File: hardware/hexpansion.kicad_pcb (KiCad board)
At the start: 2 copper layers, 86 x 45.6 mm, 87 parts, among them J1 Hexpansion-Connector, U1 AP3602AKTR-G1, U10 XL-0807RGBC-WS2812B-S, U11 XL-0807RGBC-WS2812B-S, U12 XL-0807RGBC-WS2812B-S, U13 XL-0807RGBC-WS2812B-S, U14 XL-0807RGBC-WS2812B-S, U15 XL-0807RGBC-WS2812B-S, U16 XL-0807RGBC-WS2812B-S, U17 XL-0807RGBC-WS2812B-S, U18 XL-0807RGBC-WS2812B-S, U19 XL-0807RGBC-WS2812B-S, U2 ZD24C64A-XGMT, U20 XL-0807RGBC-WS2812B-S, U21 XL-0807RGBC-WS2812B-S, U22 XL-0807RGBC-WS2812B-S, U23 XL-0807RGBC-WS2812B-S, U24 XL-0807RGBC-WS2812B-S, U25 XL-0807RGBC-WS2812B-S, U26 XL-0807RGBC-WS2812B-S, U27 XL-0807RGBC-WS2812B-S, U28 XL-0807RGBC-WS2812B-S, U29 XL-0807RGBC-WS2812B-S, U3 XL-0807RGBC-WS2812B-S, U30 XL-0807RGBC-WS2812B-S, U31 XL-0807RGBC-WS2812B-S, U32 XL-0807RGBC-WS2812B-S, U33 XL-0807RGBC-WS2812B-S, U34 XL-0807RGBC-WS2812B-S, U35 XL-0807RGBC-WS2812B-S, U36 XL-0807RGBC-WS2812B-S, U37 XL-0807RGBC-WS2812B-S, U38 XL-0807RGBC-WS2812B-S, U39 XL-0807RGBC-WS2812B-S, U4 XL-0807RGBC-WS2812B-S, U40 XL-0807RGBC-WS2812B-S, U41 XL-0807RGBC-WS2812B-S, U42 XL-0807RGBC-WS2812B-S, U43 XL-0807RGBC-WS2812B-S, U44 XL-0807RGBC-WS2812B-S, U45 XL-0807RGBC-WS2812B-S, U46 XL-0807RGBC-WS2812B-S, U47 XL-0807RGBC-WS2812B-S, U48 XL-0807RGBC-WS2812B-S, U49 XL-0807RGBC-WS2812B-S, U5 XL-0807RGBC-WS2812B-S, U50 XL-0807RGBC-WS2812B-S, U51 XL-0807RGBC-WS2812B-S, U52 XL-0807RGBC-WS2812B-S, U53 XL-0807RGBC-WS2812B-S, U54 XL-0807RGBC-WS2812B-S, U55 XL-0807RGBC-WS2812B-S, U56 XL-0807RGBC-WS2812B-S, U57 XL-0807RGBC-WS2812B-S, U58 XL-0807RGBC-WS2812B-S, U59 XL-0807RGBC-WS2812B-S, U6 XL-0807RGBC-WS2812B-S, U60 XL-0807RGBC-WS2812B-S, U61 XL-0807RGBC-WS2812B-S, U62 XL-0807RGBC-WS2812B-S, U63 XL-0807RGBC-WS2812B-S, U64 XL-0807RGBC-WS2812B-S, U65 XL-0807RGBC-WS2812B-S, U66 XL-0807RGBC-WS2812B-S, U67 XL-0807RGBC-WS2812B-S, U68 XL-0807RGBC-WS2812B-S, U69 XL-0807RGBC-WS2812B-S, U7 XL-0807RGBC-WS2812B-S, U70 XL-0807RGBC-WS2812B-S, U71 XL-0807RGBC-WS2812B-S, U72 XL-0807RGBC-WS2812B-S, U73 XL-0807RGBC-WS2812B-S, U74 XL-0807RGBC-WS2812B-S, U75 XL-0807RGBC-WS2812B-S, U76 XL-0807RGBC-WS2812B-S, U77 XL-0807RGBC-WS2812B-S, U78 XL-0807RGBC-WS2812B-S, U8 XL-0807RGBC-WS2812B-S, U9 XL-0807RGBC-WS2812B-S

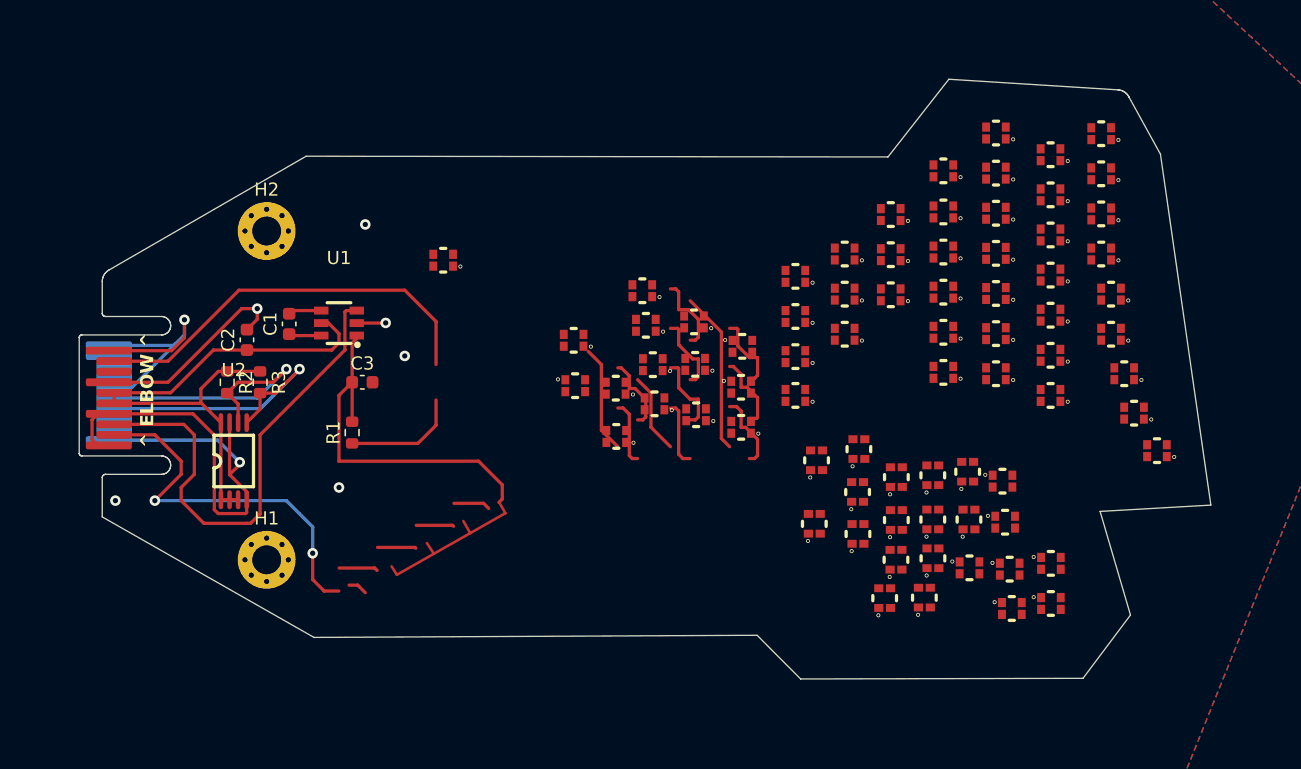
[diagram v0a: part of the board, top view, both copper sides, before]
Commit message: Fully routed
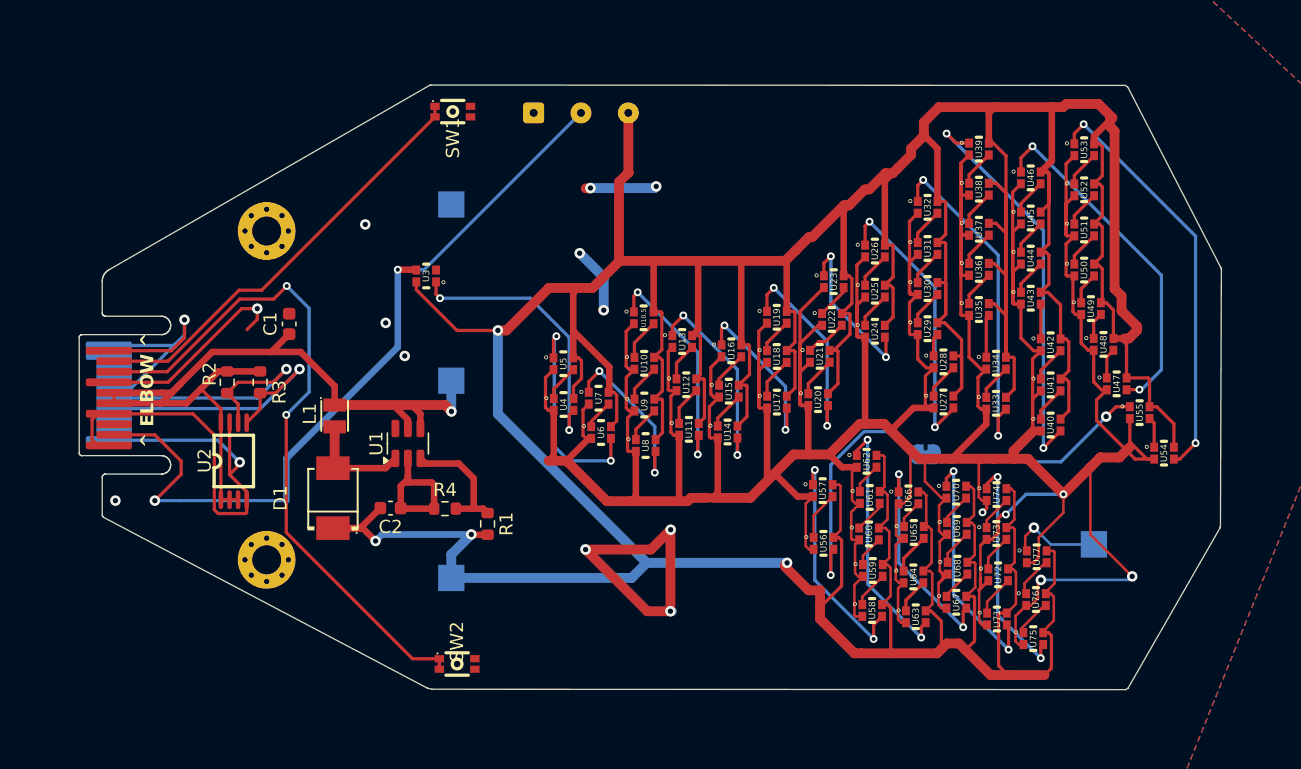
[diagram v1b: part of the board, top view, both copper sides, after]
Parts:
- removed C3: 1uF, Capacitor_SMD:C_0603_1608Metric
- added D1: SS38BF, easyeda2kicad:SMBF_L4.3-W3.6-LS5.3-RD, F.Cu at (117.5, 107.8)
- added J2: Conn_01x03_Pin, Connector_Wire:SolderWire-0.1sqmm_1x03_P3.6mm_D0.4mm_OD1mm, B.Cu at (132.8, 78.5)
- added JP1: SolderJumper_2_Bridged, Jumper:SolderJumper-2_P1.3mm_Bridged_RoundedPad1.0x1.5mm, B.Cu at (162.6, 104.5)
- added L1: AFE201610S4R7MBT, easyeda2kicad:IND-SMD_L2.0-W1.6, F.Cu at (117.7, 101.6)
- added R4: 100k, Resistor_SMD:R_0603_1608Metric, F.Cu at (126.1, 108.6)
- added SW1: SKTAACE010, easyeda2kicad:KEY-SMD_4P-L2.6-W1.6-P0.80-LS3.0, F.Cu at (126.7, 78.4)
- added SW2: SKTAACE010, easyeda2kicad:KEY-SMD_4P-L2.6-W1.6-P0.80-LS3.0, F.Cu at (127.0, 120.4)
- added TP1: TestPoint, TestPoint:TestPoint_Pad_2.0x2.0mm, B.Cu at (126.5, 98.9)
- added TP2: TestPoint, TestPoint:TestPoint_Pad_2.0x2.0mm, B.Cu at (126.5, 113.9)
- added TP3: TestPoint, TestPoint:TestPoint_Pad_2.0x2.0mm, B.Cu at (175.4, 111.3)
- added TP4: TestPoint, TestPoint:TestPoint_Pad_2.0x2.0mm, B.Cu at (126.5, 85.5)
- C1, C2: value 1uF -> 22uF
- R1: value R -> 750k
- U1: value AP3602AKTR-G1 -> MT3608; footprint easyeda2kicad:SOT-23-6_L2.9-W1.6-P0.95-LS2.8-BR -> Package_TO_SOT_SMD:SOT-23-6
- moved C2 16.8 mm to (121.9, 108.6), turned to 180 degrees
- moved U4 14.3 mm to (135.1, 100.7), turned to 0 degrees
- moved U68 13.5 mm to (165.0, 113.1), turned to 0 degrees
- moved R1 12.4 mm to (129.3, 109.8), turned to -90 degrees
- moved U3 12.2 mm to (124.6, 90.9)
- moved U1 10.5 mm to (123.2, 103.7), turned to 90 degrees
- moved U67 9.97 mm to (164.9, 115.7), turned to 0 degrees
- moved U20 9.53 mm to (154.4, 100.3), turned to 0 degrees
- moved U78 9.26 mm to (141.2, 94.1), turned to 0 degrees
- moved U11 8.56 mm to (144.6, 102.6), turned to 0 degrees
- moved U69 8.04 mm to (165.0, 110.1), turned to 0 degrees
- moved U13 7.91 mm to (144.1, 95.9), turned to 0 degrees
- moved U12 7.90 mm to (144.4, 99.2), turned to 0 degrees
- moved U61 7.72 mm to (158.4, 107.8), turned to 0 degrees
- moved U63 7.68 mm to (161.9, 116.8), turned to 0 degrees
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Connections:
- C1 pad 1: Net-(U1-C+) -> /3V3
- C1 pad 2: Net-(U1-C-) -> /GND
- C2 pad 1: /3V3 -> /GND
- C2 pad 2: /GND -> +5V
- R1 pad 1: Net-(JP1-B) -> Net-(U1-FB)
- R1 pad 2: Net-(C4-Pad1) -> +5V
- U1 pad 1: +5C -> Net-(D1-A)
- U1 pad 3: /HS_H -> Net-(U1-FB)
- U1 pad 4: Net-(U1-C-) -> /3V3
- U1 pad 6: Net-(U1-C+) -> unconnected-(U1-NC-Pad6)
- U11 pad 3: Net-(U10-DO) -> Net-(U11-DI)
- U56 pad 3: unconnected-(U56-DI-Pad3) -> Net-(JP1-B)
- U60 pad 1: unconnected-(U60-DO-Pad1) -> Net-(U60-DO)
- U61 pad 3: unconnected-(U61-DI-Pad3) -> Net-(U60-DO)
- U65 pad 1: unconnected-(U65-DO-Pad1) -> Net-(U65-DO)
- U66 pad 3: unconnected-(U66-DI-Pad3) -> Net-(U65-DO)
- U70 pad 1: unconnected-(U70-DO-Pad1) -> Net-(U70-DO)
- U71 pad 3: unconnected-(U71-DI-Pad3) -> Net-(U70-DO)
- U75 pad 1: unconnected-(U75-DO-Pad1) -> Net-(U75-DO)
- U76 pad 2: unconnected-(U76-GND-Pad2) -> /GND
- U76 pad 3: unconnected-(U76-DI-Pad3) -> Net-(U75-DO)
- U77 pad 1: unconnected-(U77-DO-Pad1) -> Net-(U77-DO)
- U77 pad 2: unconnected-(U77-GND-Pad2) -> /GND
- U78 pad 1: unconnected-(U78-DO-Pad1) -> Net-(U11-DI)
- U78 pad 2: unconnected-(U78-GND-Pad2) -> /GND
- U78 pad 3: unconnected-(U78-DI-Pad3) -> Net-(U10-DO)
- U78 pad 4: unconnected-(U78-VDD-Pad4) -> +5V
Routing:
- net +5V: track 47.2 -> 541.1 mm, vias 0 -> 4
- net /GND: track 85.0 -> 538.5 mm, vias 8 -> 19
- net Net-(J1-HS_G): track 0.00 -> 52.4 mm, vias 0 -> 2
- net /HS_H: track 37.8 -> 0.00 mm
- net /HS_I: track 28.9 -> 61.1 mm
- net Net-(U53-DO): track 0.00 -> 31.7 mm, vias 0 -> 2
- net Net-(U39-DO): track 0.00 -> 30.8 mm, vias 0 -> 2
- net /3V3: track 43.9 -> 74.3 mm, vias 0 -> 1
- net Net-(U46-DO): track 0.00 -> 26.6 mm, vias 0 -> 2
- net Net-(U32-DO): track 0.00 -> 25.9 mm, vias 0 -> 2
- net Net-(U26-DO): track 0.00 -> 21.7 mm, vias 0 -> 2
- net Net-(U62-DO): track 0.00 -> 19.5 mm, vias 0 -> 2
- net Net-(U70-DO): track 0.00 -> 18.6 mm, vias 0 -> 2
- net Net-(U57-DO): track 0.00 -> 17.9 mm, vias 0 -> 2
- net Net-(U74-DO): track 0.00 -> 17.7 mm, vias 0 -> 2
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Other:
- board size 86 x 45.6 mm -> 86.8 x 46 mm
- board text removed: "${REFERENCE}"
